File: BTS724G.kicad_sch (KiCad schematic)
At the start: 6 parts, among them U5 BTS724G

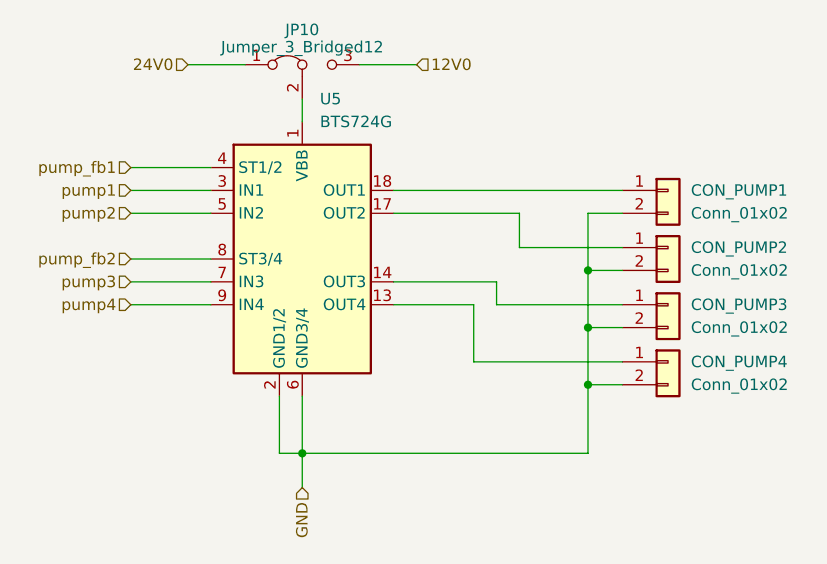
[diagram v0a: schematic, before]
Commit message: gsdfg
dyfg
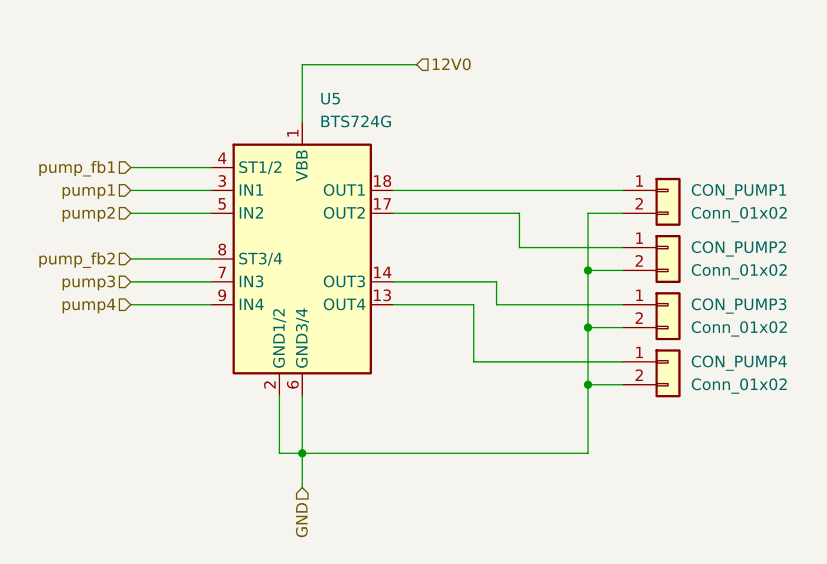
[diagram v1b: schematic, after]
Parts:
- removed JP10: Jumper_3_Bridged12, Connector_PinHeader_2.54mm:PinHeader_1x03_P2.54mm_Vertical, symbol Jumper:Jumper_3_Bridged12
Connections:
- net 12V0: now also U5.1 (VBB), U5.10 (VBB), U5.11 (VBB), U5.12 (VBB), U5.15 (VBB), U5.16 (VBB), U5.19 (VBB), U5.20 (VBB)
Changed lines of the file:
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@@
     (stroke (width 0) (type default))
   )
-  (wire (pts (xy 149.86 54.61) (xy 143.51 54.61))
+  (wire (pts (xy 137.16 54.61) (xy 149.86 54.61))
     (stroke (width 0) (type default))
   )
@@
     (stroke (width 0) (type default))
   )
-  (wire (pts (xy 137.16 58.42) (xy 137.16 60.96))
+  (wire (pts (xy 137.16 54.61) (xy 137.16 60.96))
     (stroke (width 0) (type default))
   )
@@
     (stroke (width 0) (type default))
   )
-  (wire (pts (xy 124.46 54.61) (xy 130.81 54.61))
-    (stroke (width 0) (type default))
-  )
   (wire (pts (xy 147.32 71.12) (xy 161.29 71.12))
     (stroke (width 0) (type default))
@@
   )
   (hierarchical_label "pump2" (shape input) (at 118.11 71.12 180) (fields_autoplaced)
-    (effects (font (size 1.27 1.27)) (justify right))
-  )
-  (hierarchical_label "24V0" (shape input) (at 124.46 54.61 180) (fields_autoplaced)
     (effects (font (size 1.27 1.27)) (justify right))
   )
@@
         )
       )
-    )
-  )
-  (symbol (lib_id "Jumper:Jumper_3_Bridged12") (at 137.16 54.61 0) (unit 1)
-    (in_bom yes) (on_board yes) (dnp no) (fields_autoplaced)
-    (property "Reference" "JP10" (at 137.16 50.7359 0)
-      (effects (font (size 1.27 1.27)))
-    )
-    (property "Value" "Jumper_3_Bridged12" (at 137.16 52.6569 0)
-      (effects (font (size 1.27 1.27)))
-    )
-    (property "Footprint" "Connector_PinHeader_2.54mm:PinHeader_1x03_P2.54mm_Vertical" (at 137.16 54.61 0)
-      (effects (font (size 1.27 1.27)) hide)
-    )
-    (property "Datasheet" "~" (at 137.16 54.61 0)
-      (effects (font (size 1.27 1.27)) hide)
-    )
-    (pin "1")
-    (pin "2")
-    (pin "3")
-    (instances
-      (project "rollo control"
-        (path "/7fd4875b-e2b3-49e9-a377-320ee6c6aef7/42cd8867-79f6-4c26-8217-42f6d2cc80dc"
-          (reference "JP10") (unit 1)
-        )
-        (path "/7fd4875b-e2b3-49e9-a377-320ee6c6aef7/0ae6cc60-dceb-41fc-a79b-71fa99389e9d"
-          (reference "JP6") (unit 1)
-        )
-      )
